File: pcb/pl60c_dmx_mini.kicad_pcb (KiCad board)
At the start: 4 copper layers, 38.5 x 29 mm, 37 parts, among them J1 USB-C 16P, J2 XLR-5 female (DMX OUT), Q1 S8050, SW2 BOOT, SW3 USER, U1 ESP32-S3-MINI-1-N8, U2 AP2112K-3.3, U3 SP3485EN, U4 USBLC6-2SC6

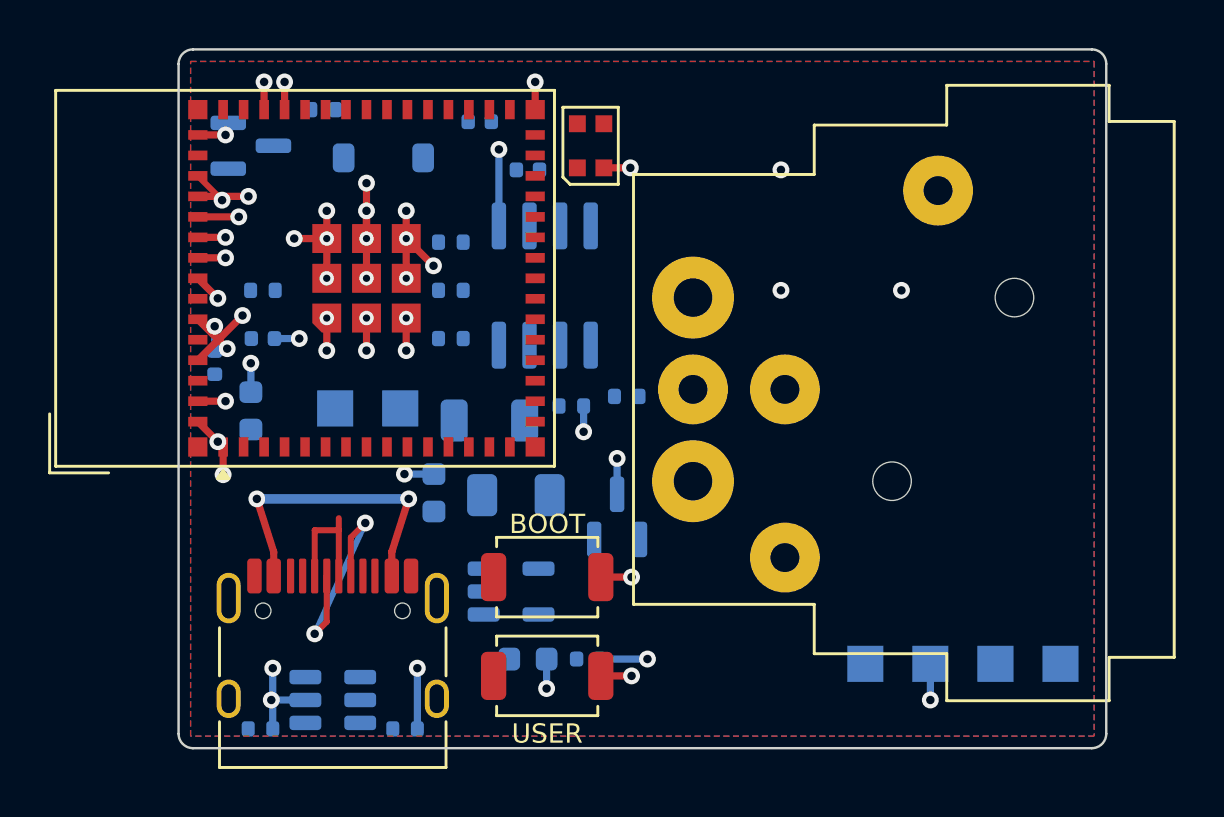
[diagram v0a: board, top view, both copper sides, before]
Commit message: auto: 2026-09-02 14:54:07
Co-Authored-By: Claude Fable 5.1 <noreply@anthropic.com>
Claude-Session: https://claude.ai/code/session_01WsrVZb94LwbHVAmBvsSTfn
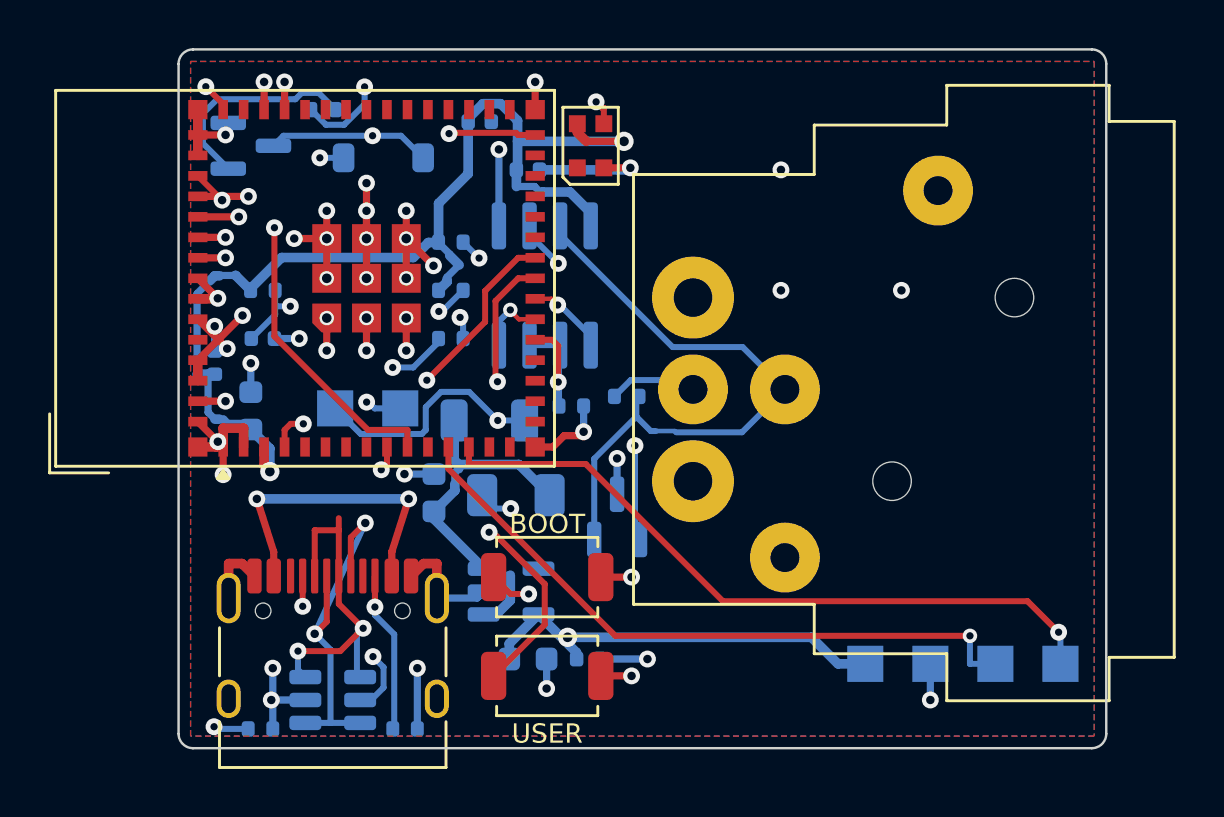
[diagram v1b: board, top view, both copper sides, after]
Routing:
- net +3V3: track 0.00 -> 87.4 mm, vias 0 -> 3
- net BZ_P: track 0.00 -> 40.1 mm, vias 0 -> 2
- net USB_D-: track 5.30 -> 38.7 mm, vias 0 -> 3
- net IO0_BOOT: track 0.00 -> 32.1 mm, vias 0 -> 3
- net EXP_SCL: track 0.00 -> 29.4 mm, vias 0 -> 1
- net EXP_SDA: track 0.00 -> 27.6 mm, vias 0 -> 1
- net DMX_B: track 0.00 -> 26.2 mm
- net USB_D+: track 10.1 -> 36.3 mm, vias 2 -> 3
- net BTN_USER: track 0.00 -> 25.7 mm, vias 0 -> 3
- net BUZZER: track 0.00 -> 23.3 mm, vias 0 -> 2
- net GND: track 63.8 -> 85.1 mm
- net DMX_A: track 0.00 -> 21.0 mm, vias 0 -> 2
- net BZ_N: track 0.00 -> 20.0 mm, vias 0 -> 2
- net LED_DATA: track 0.00 -> 17.3 mm, vias 0 -> 2
- net VBUS: track 12.9 -> 30.0 mm, vias 2 -> 4
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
